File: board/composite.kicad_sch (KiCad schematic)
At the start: 17 parts, among them J6 COMPOSITE, U17 ATF1508ASx-xxJx84, U18 74HC373, U19 74HC373, U20 74HC165, U21 74HC165, Y3 14.318 MHz

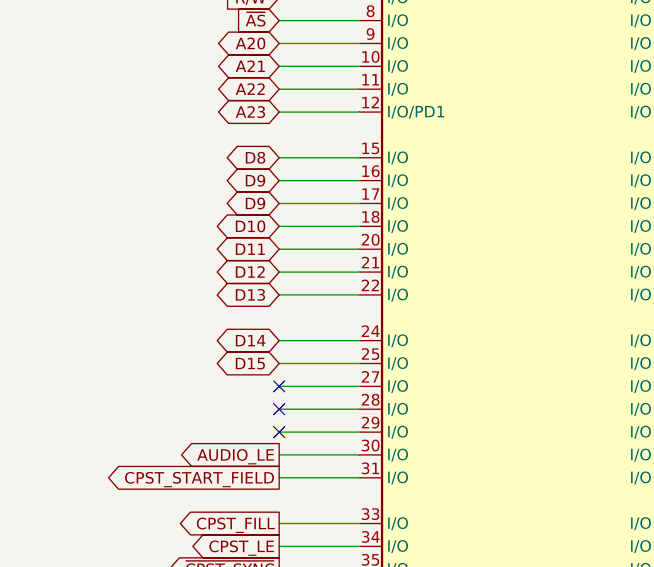
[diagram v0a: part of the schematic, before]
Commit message: design draft complete, added footprints
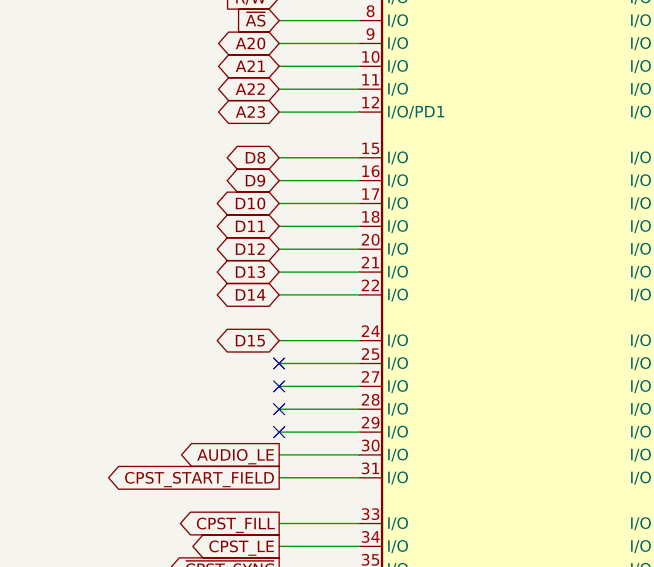
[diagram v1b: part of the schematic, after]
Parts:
- C30, C31, C32, C33, C34: footprint (none) -> Capacitor_THT:C_Disc_D5.0mm_W2.5mm_P5.00mm
- C35: footprint (none) -> Capacitor_THT:CP_Radial_D6.3mm_P2.50mm
- J6: footprint (none) -> board:CUI_RCJ-044
- R12, R14, R15, R16: footprint (none) -> Resistor_THT:R_Axial_DIN0207_L6.3mm_D2.5mm_P10.16mm_Horizontal
- U18, U19, U20, U21: footprint (none) -> Package_DIP:DIP-20_W7.62mm
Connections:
- net D10: now also U17.17 (I/O); no longer U17.18 (I/O)
- net D11: now also U17.18 (I/O); no longer U17.20 (I/O)
- net D12: now also U17.20 (I/O); no longer U17.21 (I/O)
- net D13: now also U17.21 (I/O); no longer U17.22 (I/O)
- net D14: now also U17.22 (I/O); no longer U17.24 (I/O)
- net D15: now also U17.24 (I/O); no longer U17.25 (I/O)
- net D9: no longer U17.17 (I/O)
- no-connect marks 6 -> 7
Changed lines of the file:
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@@
 	)
 	(no_connect
+		(at 50.8 124.46)
+	)
+	(no_connect
 		(at 50.8 127)
 	)
@@
 	(global_label "D13"
 		(shape bidirectional)
-		(at 50.8 116.84 180)
+		(at 50.8 114.3 180)
 		(fields_autoplaced yes)
 		(effects
@@
 		)
 		(property "Intersheetrefs" "${INTERSHEET_REFS}"
-			(at 44.224 116.84 0)
+			(at 44.224 114.3 0)
 			(effects
 				(font
@@
 		)
 	)
-	(global_label "D9"
-		(shape bidirectional)
-		(at 50.8 104.14 180)
-		(fields_autoplaced yes)
-		(effects
-			(font
-				(size 1.27 1.27)
-			)
-			(justify right)
-		)
-		(property "Intersheetrefs" "${INTERSHEET_REFS}"
-			(at 44.224 104.14 0)
-			(effects
-				(font
-					(size 1.27 1.27)
-				)
-				(justify right)
-				(hide yes)
-			)
-		)
-	)
 	(global_label "A18"
 		(shape bidirectional)
@@
 	(global_label "D14"
 		(shape bidirectional)
-		(at 50.8 121.92 180)
+		(at 50.8 116.84 180)
 		(fields_autoplaced yes)
 		(effects
@@
 		)
 		(property "Intersheetrefs" "${INTERSHEET_REFS}"
-			(at 44.224 121.92 0)
+			(at 44.224 116.84 0)
 			(effects
 				(font
@@
 	(global_label "D15"
 		(shape bidirectional)
-		(at 50.8 124.46 180)
+		(at 50.8 121.92 180)
 		(fields_autoplaced yes)
 		(effects
@@
 		)
 		(property "Intersheetrefs" "${INTERSHEET_REFS}"
-			(at 44.224 124.46 0)
+			(at 44.224 121.92 0)
 			(effects
 				(font
@@
 	(global_label "D11"
 		(shape bidirectional)
-		(at 50.8 111.76 180)
+		(at 50.8 109.22 180)
 		(fields_autoplaced yes)
 		(effects
@@
 		)
 		(property "Intersheetrefs" "${INTERSHEET_REFS}"
-			(at 44.224 111.76 0)
+			(at 44.224 109.22 0)
 			(effects
 				(font
@@
 	(global_label "D10"
 		(shape bidirectional)
-		(at 50.8 109.22 180)
+		(at 50.8 106.68 180)
 		(fields_autoplaced yes)
 		(effects
@@
 		)
 		(property "Intersheetrefs" "${INTERSHEET_REFS}"
-			(at 44.224 109.22 0)
+			(at 44.224 106.68 0)
 			(effects
 				(font
@@
 	(global_label "D9"
 		(shape bidirectional)
-		(at 50.8 106.68 180)
+		(at 50.8 104.14 180)
 		(fields_autoplaced yes)
 		(effects
@@
 		)
 		(property "Intersheetrefs" "${INTERSHEET_REFS}"
-			(at 44.224 106.68 0)
+			(at 44.224 104.14 0)
 			(effects
 				(font
@@
 	(global_label "D12"
 		(shape bidirectional)
-		(at 50.8 114.3 180)
+		(at 50.8 111.76 180)
 		(fields_autoplaced yes)
 		(effects
@@
 		)
 		(property "Intersheetrefs" "${INTERSHEET_REFS}"
-			(at 44.224 114.3 0)
+			(at 44.224 111.76 0)
 			(effects
 				(font
@@
 			)
 		)
-		(property "Footprint" ""
+		(property "Footprint" "Package_DIP:DIP-20_W7.62mm"
 			(at 195.58 63.5 0)
 			(effects
@@
 			)
 		)
-		(property "Footprint" ""
+		(property "Footprint" "Capacitor_THT:CP_Radial_D6.3mm_P2.50mm"
 			(at 314.96 101.9048 0)
 			(effects
@@
 			)
 		)
-		(property "Footprint" ""
+		(property "Footprint" "Resistor_THT:R_Axial_DIN0207_L6.3mm_D2.5mm_P10.16mm_Horizontal"
 			(at 295.91 113.538 90)
 			(effects
@@
 			)
 		)
-		(property "Footprint" ""
+		(property "Footprint" "Capacitor_THT:C_Disc_D5.0mm_W2.5mm_P5.00mm"
 			(at 67.0052 193.04 0)
 			(effects
@@
 			)
 		)
-		(property "Footprint" ""
+		(property "Footprint" "Resistor_THT:R_Axial_DIN0207_L6.3mm_D2.5mm_P10.16mm_Horizontal"
 			(at 327.66 104.648 90)
 			(effects
@@
 			)
 		)
-		(property "Footprint" ""
+		(property "Footprint" "Capacitor_THT:C_Disc_D5.0mm_W2.5mm_P5.00mm"
 			(at 155.9052 88.9 0)
 			(effects
@@
 			)
 		)
-		(property "Footprint" ""
+		(property "Footprint" "Package_DIP:DIP-20_W7.62mm"
 			(at 231.14 127 0)
 			(effects
@@
 			)
 		)
-		(property "Footprint" ""
+		(property "Footprint" "Package_DIP:DIP-20_W7.62mm"
 			(at 231.14 63.5 0)
 			(effects
@@
 			)
 		)
-		(property "Footprint" ""
+		(property "Footprint" "board:CUI_RCJ-044"
 			(at 345.44 102.87 0)
 			(effects
@@
 			)
 		)
-		(property "Footprint" ""
+		(property "Footprint" "Capacitor_THT:C_Disc_D5.0mm_W2.5mm_P5.00mm"
 			(at 197.8152 172.72 0)
 			(effects
@@
 			)
 		)
-		(property "Footprint" ""
+		(property "Footprint" "Package_DIP:DIP-20_W7.62mm"
 			(at 195.58 127 0)
 			(effects
@@
 			)
 		)
-		(property "Footprint" ""
+		(property "Footprint" "Resistor_THT:R_Axial_DIN0207_L6.3mm_D2.5mm_P10.16mm_Horizontal"
 			(at 295.91 98.298 90)
 			(effects
@@
 			)
 		)
-		(property "Footprint" ""
+		(property "Footprint" "Capacitor_THT:C_Disc_D5.0mm_W2.5mm_P5.00mm"
 			(at 155.9052 148.59 0)
 			(effects
@@
 			)
 		)
-		(property "Footprint" ""
+		(property "Footprint" "Resistor_THT:R_Axial_DIN0207_L6.3mm_D2.5mm_P10.16mm_Horizontal"
 			(at 22.352 29.21 90)
 			(effects
@@
 			)
 		)
-		(property "Footprint" ""
+		(property "Footprint" "Capacitor_THT:C_Disc_D5.0mm_W2.5mm_P5.00mm"
 			(at 178.7652 172.72 0)
 			(effects
